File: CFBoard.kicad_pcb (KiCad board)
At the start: 2 copper layers, 80 x 60 mm, 21 parts, among them U1 STM32 Blue Pill, U2 Wemos D1 Mini, U3 GY-6500, U4 BMP180_5pin

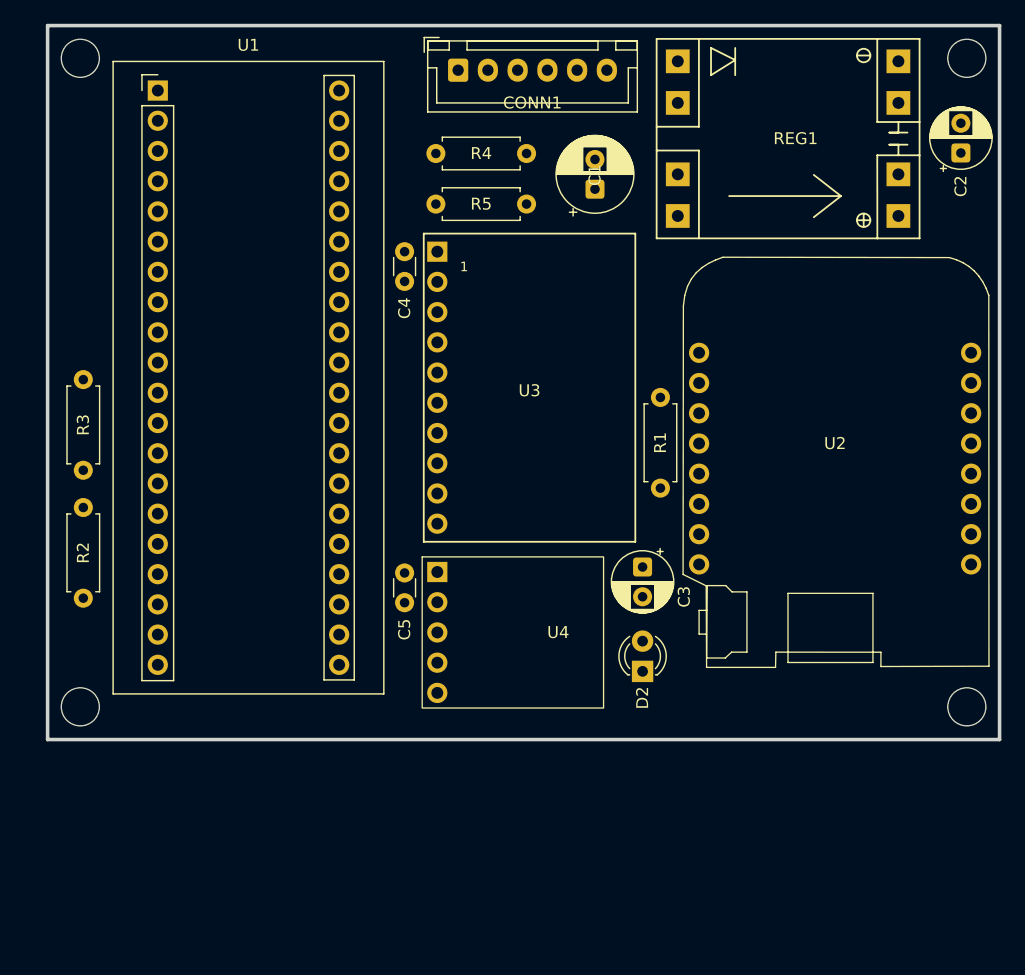
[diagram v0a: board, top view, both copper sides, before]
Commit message: feat: wrap up version 1
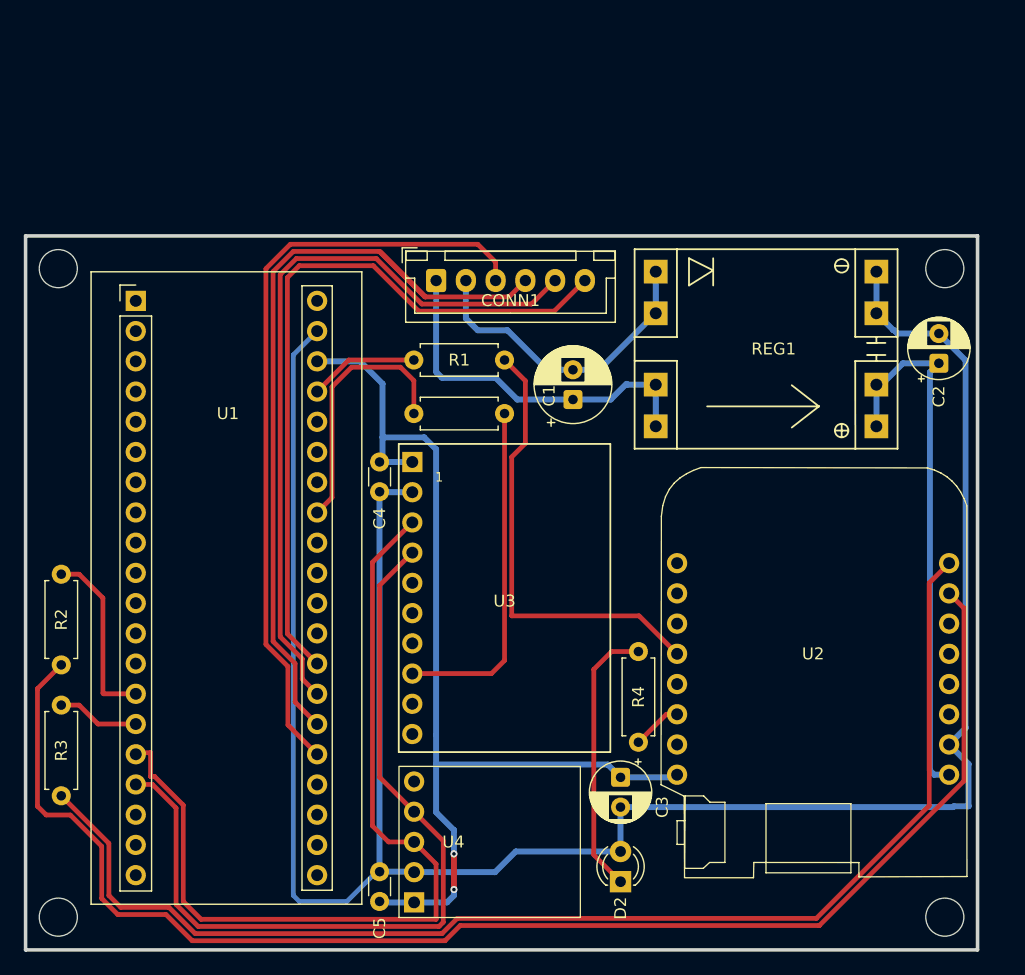
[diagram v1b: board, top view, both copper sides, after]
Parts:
- moved R4 45.2 mm to (159.6, 113.2), turned to -90 degrees
- moved R3 27.4 mm to (111.1, 117.7)
- moved C5 25.2 mm to (137.9, 131.7)
- moved R5 18.5 mm to (148.4, 93.2), turned to 180 degrees
- moved C4 17.8 mm to (137.9, 97.2)
- moved U3 17.8 mm to (148.4, 108.7)
- moved REG1 17.8 mm to (170.4, 87.7)
- moved C1 17.8 mm to (154.1, 92.0)
- moved C3 17.8 mm to (158.1, 123.7)
- moved CONN1 17.8 mm to (142.6, 82.0)
- moved REF** 17.8 mm to (185.4, 81.0)
- moved REF** 17.8 mm to (110.9, 81.0)
- moved C2 17.8 mm to (184.9, 89.0)
- moved D2 17.8 mm to (158.1, 132.5)
- moved REF** 17.8 mm to (110.9, 135.5)
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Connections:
- C5 pad 1: Net-(U2-3.3V) -> Net-(D2-A)
- C5 pad 2: Net-(D2-A) -> Net-(U2-3.3V)
- R5 pad 1: Net-(U1-PB9) -> Net-(U3-INT)
- U3 pad 8: Net-(U1-PB9) -> Net-(U3-INT)
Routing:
- net Net-(D2-A): track 0.00 -> 196.8 mm
- net Net-(U2-Rx): track 0.00 -> 119.7 mm
- net Net-(U2-Tx): track 0.00 -> 105.8 mm
- net Net-(U2-3.3V): track 0.00 -> 85.8 mm, vias 0 -> 2
- net Net-(U1-PB8): track 0.00 -> 75.6 mm
- net Net-(U1-PB9): track 0.00 -> 70.1 mm
- net Net-(CONN1-Signal_2): track 0.00 -> 69.0 mm
- net Net-(CONN1-Signal_1): track 0.00 -> 64.9 mm
- net Net-(CONN1-Signal_3): track 0.00 -> 62.6 mm
- net Net-(CONN1-Signal_4): track 0.00 -> 61.5 mm
- net Net-(REG1-VOUT+): track 0.00 -> 46.4 mm
- net Net-(U2-D5): track 0.00 -> 37.9 mm
- net Net-(CONN1-VIN): track 0.00 -> 31.5 mm
- net Net-(U3-INT): track 0.00 -> 29.0 mm
- net Net-(CONN1-GND): track 0.00 -> 26.5 mm
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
